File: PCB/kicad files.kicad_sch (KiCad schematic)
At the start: 0 parts

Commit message: microcotroler schema
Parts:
- added SW1, SW2, SW3: SW_Push, symbol Switch:SW_Push
- added U1: MOUDLE-SEEEDUINO-XIAO, symbol XIAO_RP2040:MOUDLE-SEEEDUINO-XIAO
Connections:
- new net: SW3.1, U1.9 (PA7_A8_D8_SCK)
- new net: SW1.1, U1.11 (PA6_A10_D10_MOSI)
- new net: SW2.1, U1.10 (PA5_A9_D9_MISO)
- new net GND: SW1.2, SW2.2, SW3.2, U1.13 (GND)

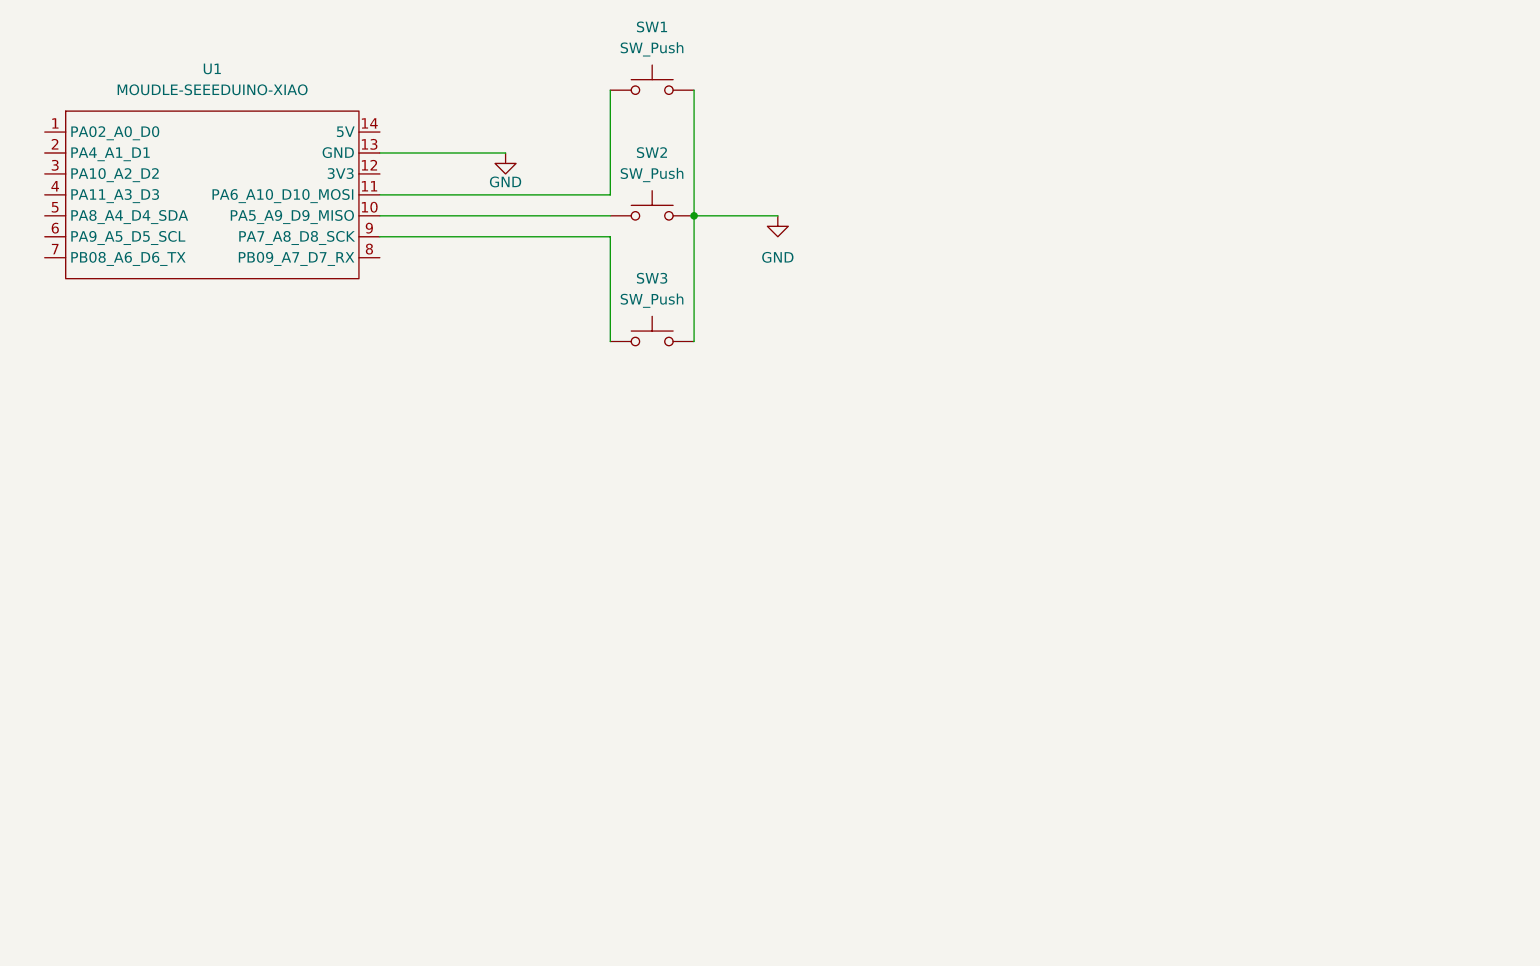
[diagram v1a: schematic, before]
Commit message: switch and diode schema
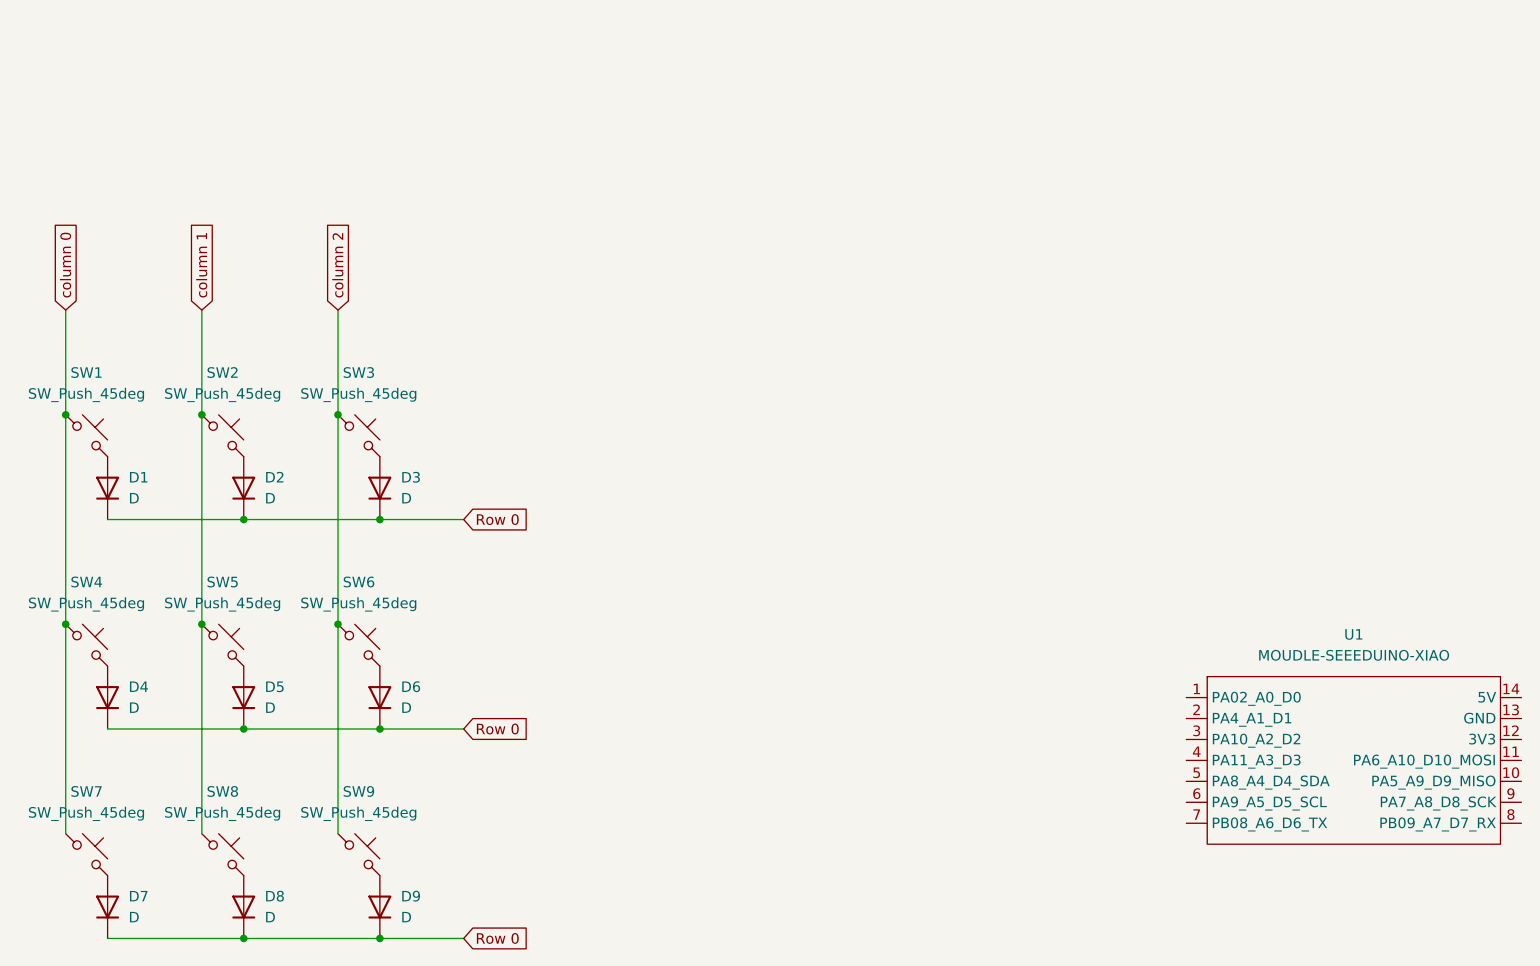
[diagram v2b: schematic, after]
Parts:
- removed SW1, SW2, SW3: SW_Push, symbol Switch:SW_Push
- added D1, D2, D3, D4, D5, D6, D7, D8, D9: D, symbol Device:D
- added SW1, SW2, SW3, SW4, SW5, SW6, SW7, SW8, SW9: SW_Push_45deg, symbol Switch:SW_Push_45deg
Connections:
- net GND: no longer names the net of U1.13 (GND)
- new net: D2.2 (A), SW2.2
- new net: D5.2 (A), SW5.2
- new net: D1.2 (A), SW1.2
- new net: D4.2 (A), SW4.2
- new net: D8.2 (A), SW8.2
- new net: D9.2 (A), SW9.2
- new net: D3.2 (A), SW3.2
- new net: D6.2 (A), SW6.2
- new net: D7.2 (A), SW7.2
- new net Row 0: D1.1 (K), D2.1 (K), D3.1 (K), D4.1 (K), D5.1 (K), D6.1 (K), D7.1 (K), D8.1 (K), D9.1 (K)
- new net column 0: SW1.1, SW4.1, SW7.1
- new net column 1: SW2.1, SW5.1, SW8.1
- new net column 2: SW3.1, SW6.1, SW9.1
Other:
- moved on the sheet: U1
